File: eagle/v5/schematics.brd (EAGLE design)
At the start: 73.6 x 41.6 mm, 25 parts, among them T1 MMBT2222A, U1 SN74LVC2G14

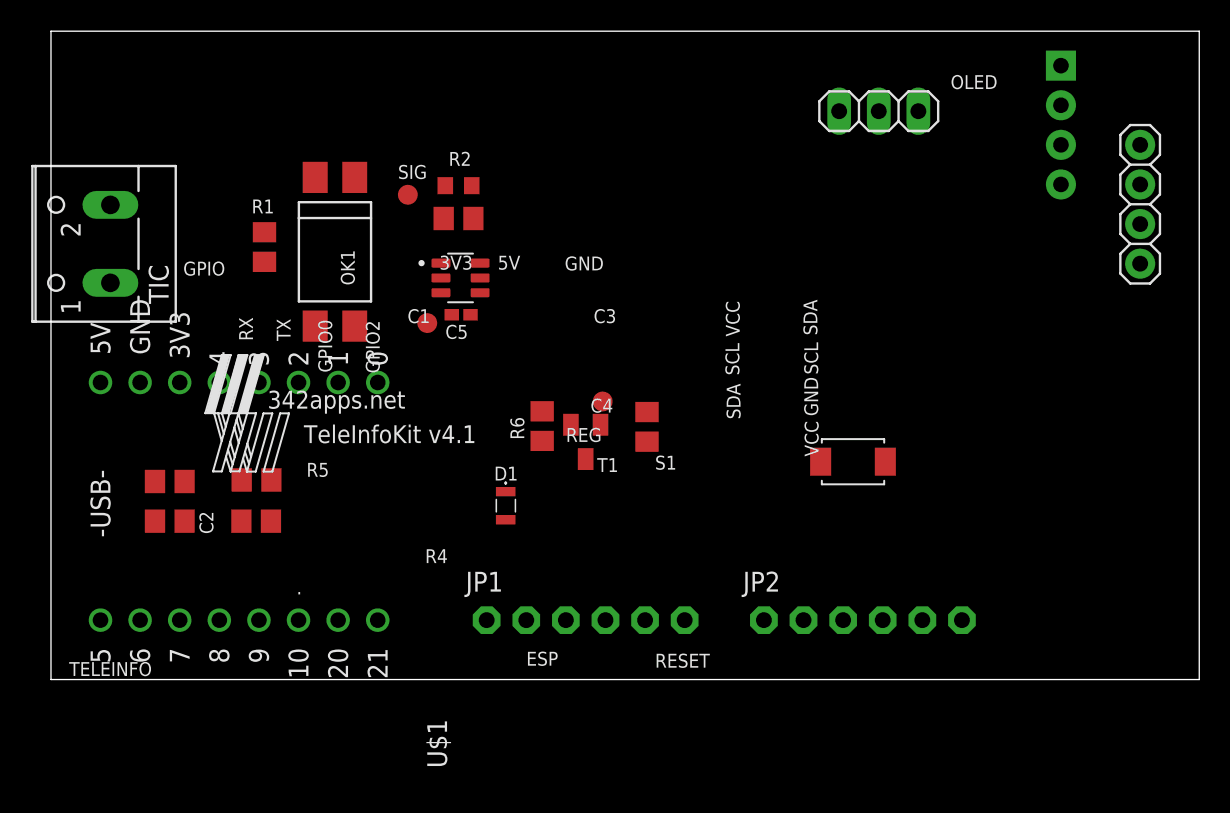
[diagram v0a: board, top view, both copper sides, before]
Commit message: V5 update
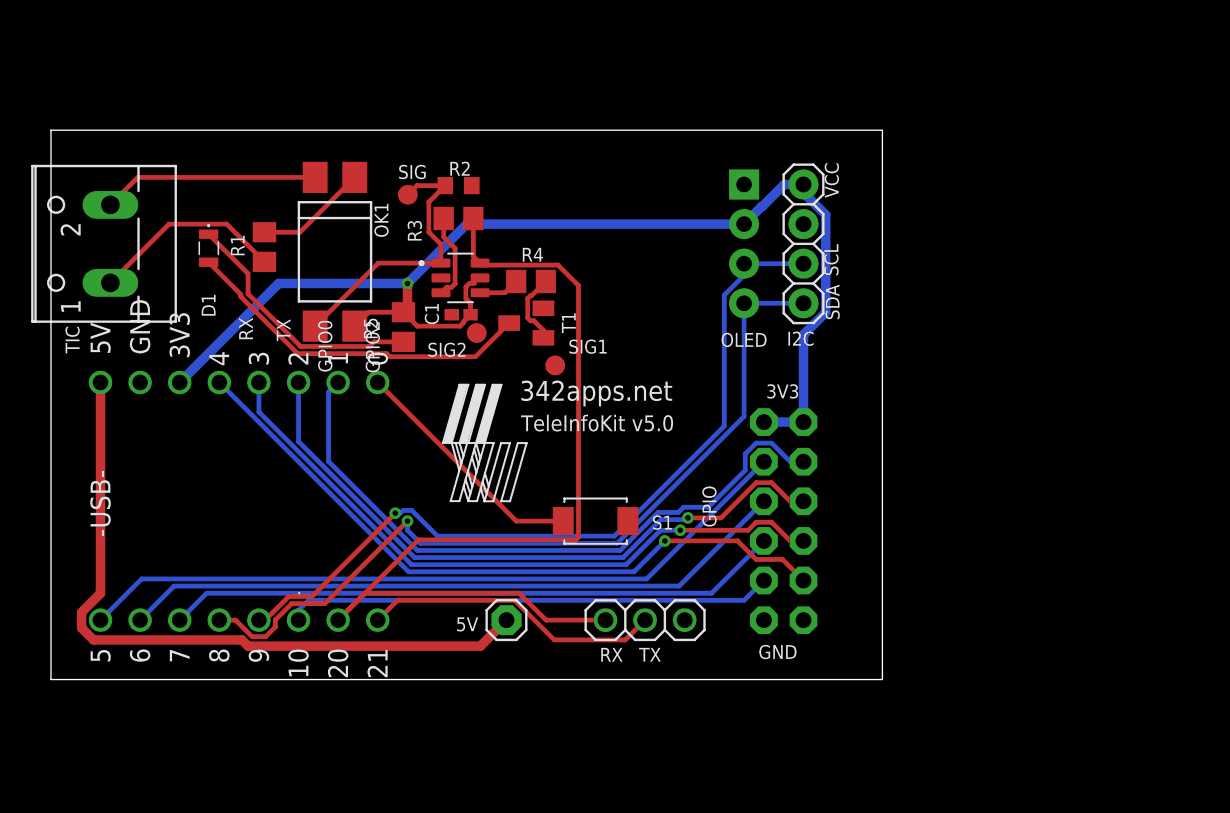
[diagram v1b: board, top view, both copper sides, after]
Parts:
- removed C2, C4: 1uF, rcl:C0805
- removed C3: 4.7uF, rcl:C0805
- removed C5: 0.1uF, rcl:C0402K
- removed POWER: (no value), pinhead:1X03
- removed R6: 300, rcl:R0805
- added 5V: (no value), adafruit:1X01
- added JP3: (no value), adafruit:1X03
- added R3: 1k, rcl:R0805
- C1: value 4.7uF -> 0.1uF; device rcl:C0805 -> rcl:C0402K
- R4: value 1k -> 10k
- R5: value 10k -> 300
- moved D1 25.2 mm to (10.1, 27.7)
- moved I2C 21.7 mm to (48.3, 27.9), turned to 90 degrees
- moved OLED 21.7 mm to (26.7, 27.9)
- moved C1 21.5 mm to (26.3, 23.4)
- moved S1 16.9 mm to (34.9, 10.2)
- moved R5 16.9 mm to (22.6, 22.6)
- moved JP1 13.1 mm to (45.7, 10.2), turned to 90 degrees
- moved T1 8.52 mm to (30.5, 22.9), turned to 90 degrees
- moved JP2 7.41 mm to (48.3, 10.2), turned to 90 degrees
- moved R4 6.16 mm to (30.8, 25.5)
- moved SIG1 3.83 mm to (32.3, 20.1), turned to 90 degrees
- moved SIG2 3.24 mm to (27.3, 22.2)
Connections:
- net +3V3: now also C1.1, R5.1; no longer C3.1, C4.1, C5.1, POWER.1, R6.1
- net +5V: now also 5V.1; no longer C1.1, C2.1, POWER.2
- net GND: now also JP3.1; no longer C2.2, C3.2, C4.2, C5.2, POWER.3
- net N$13: now also R4.2; no longer R5.2
- net N$15: now also R3.1; no longer R4.1
- net N$3: now also R5.2; no longer R6.2
- net N$5: now also R4.1; no longer R5.1
- net RXD: now also JP3.3, R3.2; no longer R4.2
- net TXD: now also JP3.2
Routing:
- net +3V3: track 0.00 -> 77.2 mm, vias 0 -> 1
- net RXD: track 0.00 -> 62.3 mm
- net N$2: track 0.00 -> 52.8 mm, vias 0 -> 1
- net N$6: track 0.00 -> 51.1 mm, vias 0 -> 1
- net N$10: track 0.00 -> 46.8 mm
- net +5V: track 0.00 -> 44.7 mm
- net N$18: track 0.00 -> 44.4 mm, vias 0 -> 1
- net N$14: track 0.00 -> 43.2 mm
- net N$19: track 0.00 -> 42.5 mm, vias 0 -> 1
- net N$21: track 0.00 -> 42.1 mm
- net N$20: track 0.00 -> 41.7 mm, vias 0 -> 1
- net N$16: track 0.00 -> 39.6 mm
- net N$17: track 0.00 -> 31.3 mm
- net N$12: track 0.00 -> 22.8 mm
- net TXD: track 0.00 -> 19.2 mm
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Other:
- board size 73.6 x 41.6 mm -> 53.3 x 35.2 mm
- board text added: "TeleInfoKit v5.0"
- board text removed: "C1"
- board text removed: "C3"
- board text removed: "C4"
- board text removed: "ESP"
- board text removed: "OLED"
- board text removed: "R4"
- board text removed: "R5"
- board text removed: "REG"
- board text removed: "RESET"
- board text removed: "S1"
- board text removed: "TELEINFO"
